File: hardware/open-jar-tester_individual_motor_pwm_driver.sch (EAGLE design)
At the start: 6 parts

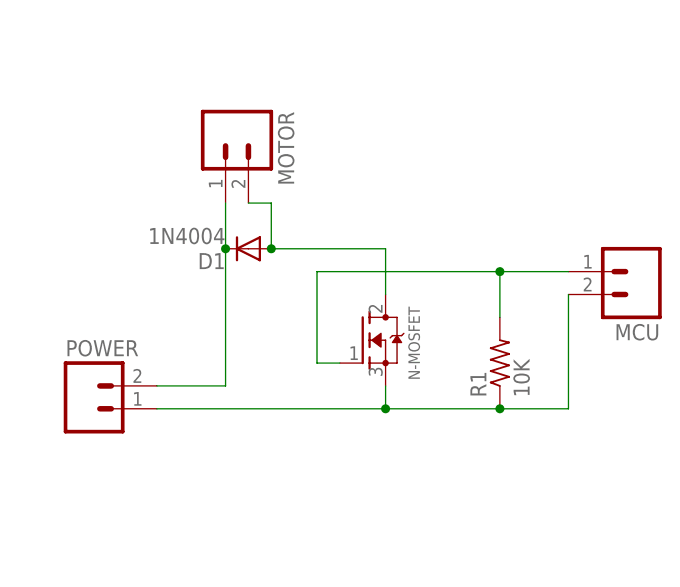
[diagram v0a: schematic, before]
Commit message: deleting temp files
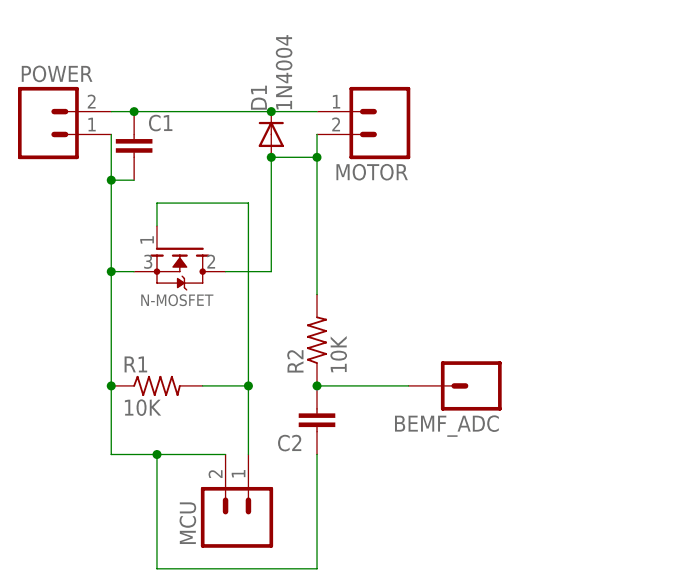
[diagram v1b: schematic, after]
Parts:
- added BEMF_ADC: (no value), SparkFun-Connectors:M01PTH
- added C1, C2: (no value), SparkFun-Passives:CAPPTH
- added R2: 10K, adafruit:R-US_0207/10
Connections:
- new net N$1: BEMF_ADC.1, C2.2, R2.1
- net GND: now also C1.2, C2.1
- net N$3: now also R2.2
- net N$4: now also C1.1
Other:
- moved on the sheet: D1, MCU, MOTOR, N-MOSFET, POWER, R1
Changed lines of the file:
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@@
 <setting verticaltext="up"/>
 </settings>
-<grid distance="0.05" unitdist="inch" unit="inch" style="lines" multiple="1" display="no" altdistance="0.01" altunitdist="inch" altunit="inch"/>
+<grid distance="0.1" unitdist="inch" unit="inch" style="lines" multiple="1" display="no" altdistance="0.01" altunitdist="inch" altunit="inch"/>
 <layers>
 <layer number="1" name="Top" color="4" fill="1" visible="no" active="no"/>
@@
 <part name="R1" library="adafruit" deviceset="R-US_" device="0207/10" value="10K"/>
 <part name="D1" library="diode" deviceset="1N4004" device=""/>
+<part name="C1" library="SparkFun-Passives" deviceset="CAP" device="PTH"/>
+<part name="R2" library="adafruit" deviceset="R-US_" device="0207/10" value="10K"/>
+<part name="C2" library="SparkFun-Passives" deviceset="CAP" device="PTH"/>
+<part name="BEMF_ADC" library="SparkFun-Connectors" deviceset="M01" device="PTH"/>
 </parts>
 <sheets>
@@
 </plain>
 <instances>
-<instance part="N-MOSFET" gate="G$1" x="30.48" y="25.4" smashed="yes">
-<attribute name="NAME" x="36.83" y="20.955" size="1.27" layer="95" rot="R90"/>
-<attribute name="VALUE" x="35.56" y="24.13" size="1.27" layer="96"/>
+<instance part="N-MOSFET" gate="G$1" x="10.16" y="35.56" smashed="yes" rot="R270">
+<attribute name="NAME" x="5.715" y="29.21" size="1.27" layer="95"/>
+<attribute name="VALUE" x="8.89" y="30.48" size="1.27" layer="96" rot="R270"/>
 </instance>
-<instance part="POWER" gate="G$1" x="0" y="17.78"/>
-<instance part="MOTOR" gate="G$1" x="15.24" y="48.26" rot="R270"/>
-<instance part="MCU" gate="G$1" x="60.96" y="33.02" rot="R180"/>
-<instance part="R1" gate="G$1" x="45.72" y="22.86" rot="R90"/>
-<instance part="D1" gate="1" x="17.78" y="35.56" rot="R180"/>
+<instance part="POWER" gate="G$1" x="-5.08" y="48.26"/>
+<instance part="MOTOR" gate="G$1" x="33.02" y="50.8" rot="R180"/>
+<instance part="MCU" gate="G$1" x="17.78" y="5.08" rot="R90"/>
+<instance part="R1" gate="G$1" x="7.62" y="20.32"/>
+<instance part="D1" gate="1" x="20.32" y="48.26" rot="R90"/>
+<instance part="C1" gate="G$1" x="5.08" y="45.72"/>
+<instance part="R2" gate="G$1" x="25.4" y="25.4" rot="R90"/>
+<instance part="C2" gate="G$1" x="25.4" y="17.78" rot="R180"/>
+<instance part="BEMF_ADC" gate="G$1" x="43.18" y="20.32" rot="R180"/>
 </instances>
 <busses>
@@
 <net name="N$2" class="0">
 <segment>
-<wire x1="25.4" y1="33.02" x2="25.4" y2="22.86" width="0.1524" layer="91"/>
+<wire x1="17.78" y1="40.64" x2="7.62" y2="40.64" width="0.1524" layer="91"/>
 <pinref part="N-MOSFET" gate="G$1" pin="G"/>
-<wire x1="25.4" y1="22.86" x2="27.94" y2="22.86" width="0.1524" layer="91"/>
+<wire x1="7.62" y1="40.64" x2="7.62" y2="38.1" width="0.1524" layer="91"/>
 <pinref part="MCU" gate="G$1" pin="1"/>
-<wire x1="53.34" y1="33.02" x2="45.72" y2="33.02" width="0.1524" layer="91"/>
+<wire x1="17.78" y1="12.7" x2="17.78" y2="20.32" width="0.1524" layer="91"/>
 <pinref part="R1" gate="G$1" pin="2"/>
-<wire x1="45.72" y1="33.02" x2="45.72" y2="27.94" width="0.1524" layer="91"/>
-<wire x1="25.4" y1="33.02" x2="45.72" y2="33.02" width="0.1524" layer="91"/>
-<junction x="45.72" y="33.02"/>
+<wire x1="17.78" y1="20.32" x2="12.7" y2="20.32" width="0.1524" layer="91"/>
+<wire x1="17.78" y1="40.64" x2="17.78" y2="20.32" width="0.1524" layer="91"/>
+<junction x="17.78" y="20.32"/>
 </segment>
 </net>
@@
 <segment>
 <pinref part="MOTOR" gate="G$1" pin="1"/>
-<wire x1="15.24" y1="40.64" x2="15.24" y2="35.56" width="0.1524" layer="91"/>
+<wire x1="25.4" y1="50.8" x2="20.32" y2="50.8" width="0.1524" layer="91"/>
 <pinref part="POWER" gate="G$1" pin="2"/>
-<wire x1="15.24" y1="35.56" x2="15.24" y2="20.32" width="0.1524" layer="91"/>
-<wire x1="15.24" y1="20.32" x2="7.62" y2="20.32" width="0.1524" layer="91"/>
+<wire x1="20.32" y1="50.8" x2="5.08" y2="50.8" width="0.1524" layer="91"/>
 <pinref part="D1" gate="1" pin="C"/>
-<junction x="15.24" y="35.56"/>
+<junction x="20.32" y="50.8"/>
+<pinref part="C1" gate="G$1" pin="1"/>
+<wire x1="5.08" y1="50.8" x2="2.54" y2="50.8" width="0.1524" layer="91"/>
+<junction x="5.08" y="50.8"/>
 </segment>
 </net>
@@
 <segment>
 <pinref part="MOTOR" gate="G$1" pin="2"/>
-<wire x1="17.78" y1="40.64" x2="20.32" y2="40.64" width="0.1524" layer="91"/>
+<wire x1="25.4" y1="48.26" x2="25.4" y2="45.72" width="0.1524" layer="91"/>
 <pinref part="D1" gate="1" pin="A"/>
-<wire x1="20.32" y1="40.64" x2="20.32" y2="35.56" width="0.1524" layer="91"/>
-<wire x1="20.32" y1="35.56" x2="33.02" y2="35.56" width="0.1524" layer="91"/>
-<junction x="20.32" y="35.56"/>
+<wire x1="25.4" y1="45.72" x2="20.32" y2="45.72" width="0.1524" layer="91"/>
+<wire x1="20.32" y1="45.72" x2="20.32" y2="33.02" width="0.1524" layer="91"/>
+<junction x="20.32" y="45.72"/>
 <pinref part="N-MOSFET" gate="G$1" pin="D"/>
-<wire x1="33.02" y1="35.56" x2="33.02" y2="30.48" width="0.1524" layer="91"/>
+<wire x1="20.32" y1="33.02" x2="15.24" y2="33.02" width="0.1524" layer="91"/>
+<wire x1="25.4" y1="45.72" x2="25.4" y2="30.48" width="0.1524" layer="91"/>
+<junction x="25.4" y="45.72"/>
+<pinref part="R2" gate="G$1" pin="2"/>
 </segment>
 </net>
@@
 <segment>
 <pinref part="POWER" gate="G$1" pin="1"/>
-<wire x1="7.62" y1="17.78" x2="33.02" y2="17.78" width="0.1524" layer="91"/>
+<wire x1="2.54" y1="48.26" x2="2.54" y2="43.18" width="0.1524" layer="91"/>
 <pinref part="MCU" gate="G$1" pin="2"/>
-<wire x1="33.02" y1="17.78" x2="45.72" y2="17.78" width="0.1524" layer="91"/>
-<wire x1="45.72" y1="17.78" x2="53.34" y2="17.78" width="0.1524" layer="91"/>
-<wire x1="53.34" y1="17.78" x2="53.34" y2="30.48" width="0.1524" layer="91"/>
+<wire x1="2.54" y1="43.18" x2="2.54" y2="33.02" width="0.1524" layer="91"/>
+<wire x1="2.54" y1="33.02" x2="2.54" y2="20.32" width="0.1524" layer="91"/>
+<wire x1="2.54" y1="20.32" x2="2.54" y2="12.7" width="0.1524" layer="91"/>
+<wire x1="2.54" y1="12.7" x2="7.62" y2="12.7" width="0.1524" layer="91"/>
 <pinref part="N-MOSFET" gate="G$1" pin="S"/>
-<wire x1="33.02" y1="20.32" x2="33.02" y2="17.78" width="0.1524" layer="91"/>
-<junction x="33.02" y="17.78"/>
+<wire x1="7.62" y1="12.7" x2="15.24" y2="12.7" width="0.1524" layer="91"/>
+<wire x1="5.08" y1="33.02" x2="2.54" y2="33.02" width="0.1524" layer="91"/>
+<junction x="2.54" y="33.02"/>
 <pinref part="R1" gate="G$1" pin="1"/>
-<junction x="45.72" y="17.78"/>
-</segment>
-</net>
+<junction x="2.54" y="20.32"/>
+<pinref part="C1" gate="G$1" pin="2"/>
+<wire x1="5.08" y1="43.18" x2="2.54" y2="43.18" width="0.1524" layer="91"/>
+<junction x="2.54" y="43.18"/>
+<pinref part="C2" gate="G$1" pin="1"/>
+<wire x1="25.4" y1="0" x2="25.4" y2="12.7" width="0.1524" layer="91"/>
+<wire x1="7.62" y1="0" x2="25.4" y2="0" width="0.1524" layer="91"/>
+<wire x1="7.62" y1="0" x2="7.62" y2="12.7" width="0.1524" layer="91"/>
+<junction x="7.62" y="12.7"/>
+</segment>
+</net>
+<net name="N$1" class="0">
+<segment>
+<pinref part="R2" gate="G$1" pin="1"/>
+<pinref part="C2" gate="G$1" pin="2"/>
+<wire x1="35.56" y1="20.32" x2="25.4" y2="20.32" width="0.1524" layer="91"/>
+<junction x="25.4" y="20.32"/>
+<pinref part="BEMF_ADC" gate="G$1" pin="1"/>
+</segment>
+</net>
